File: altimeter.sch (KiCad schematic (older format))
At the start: 23 parts, among them J1 Conn_01x03_Male, J2 Conn_01x05_Male, J3 Conn_01x05_Male, J4 Conn_01x03_Male, Q1 Q_NMOS_DGS, U1 TLV760, U2 test, U3 accel, U4 RN4871, U5 EEPROM, U6 BMP280

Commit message: wip
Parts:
- removed C6: 1u, Capacitors_SMD:C_0805_HandSoldering, symbol CP
- removed J4: Conn_01x03_Male, Pin_Headers:Pin_Header_Straight_1x03_Pitch2.54mm, symbol Conn_01x03_Male
- removed Q1: Q_NMOS_DGS, TO_SOT_Packages_SMD:SOT-23, symbol Q_NMOS_DGS
- removed R4: 100k, Resistors_SMD:R_0805_HandSoldering, symbol R
- removed R5: 5, Resistors_SMD:R_0805_HandSoldering, symbol R
- removed U3: accel, SMD_Packages:SOIC-8-N, symbol accel
- removed U5: EEPROM, lib:SO8, symbol EEPROM
- C1, C2, C3, C4, C5, C7: footprint Capacitors_SMD:C_0805_HandSoldering -> Capacitors_SMD:C_0603
- J2, J3: footprint Pin_Headers:Pin_Header_Straight_1x05_Pitch2.54mm -> lib:pin5
- R1, R2, R3: footprint Resistors_SMD:R_0805_HandSoldering -> Resistors_SMD:R_0603
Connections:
- wire segments 119 -> 82

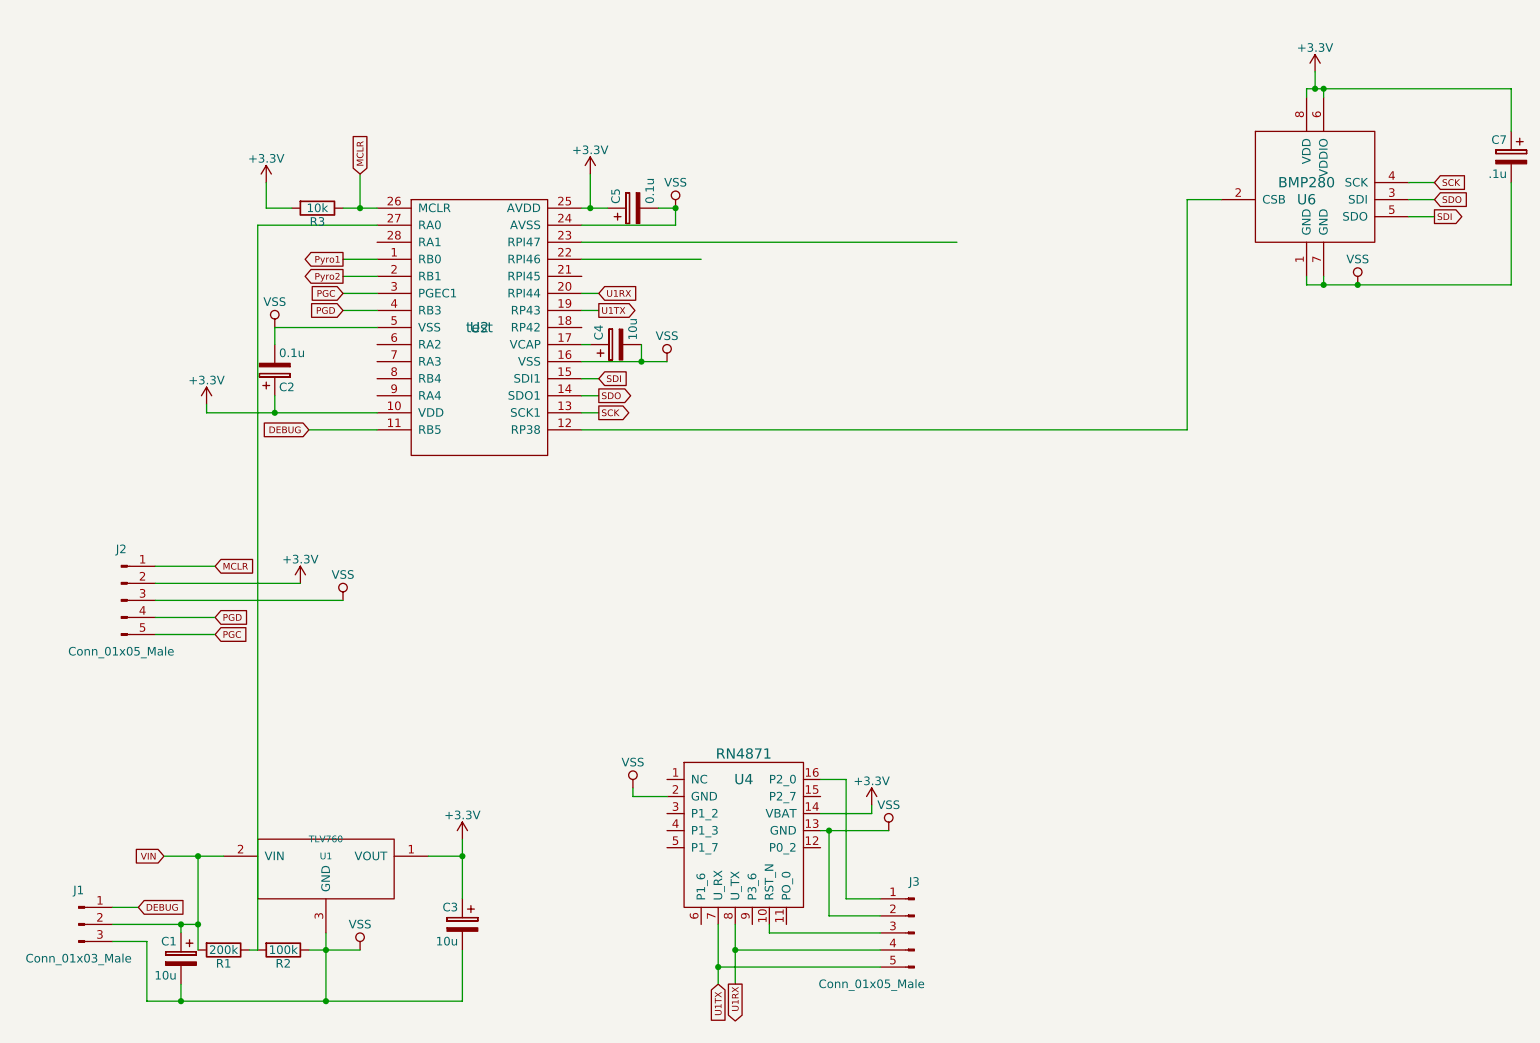
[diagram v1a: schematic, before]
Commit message: wip
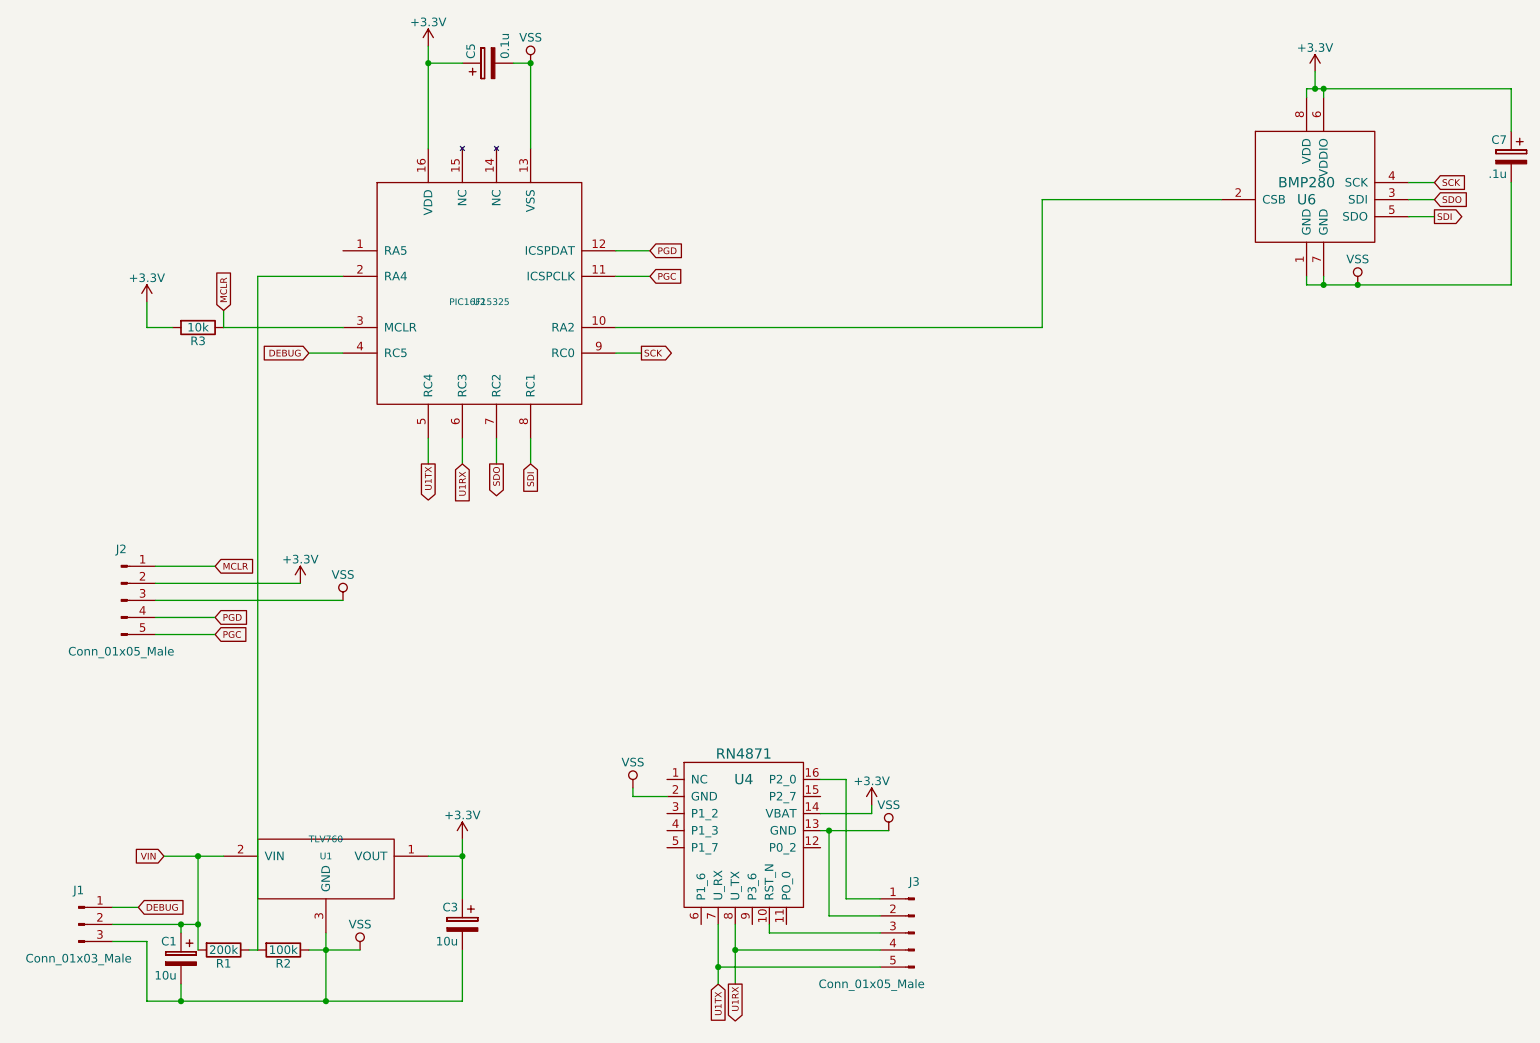
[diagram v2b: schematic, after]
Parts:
- removed C2: 0.1u, Capacitors_SMD:C_0603, symbol CP
- removed C4: 10u, Capacitors_SMD:C_0603, symbol CP
- removed U2: test, lib:QFN_28, symbol dsPIC33_qfn
- added U2: PIC16F15325, symbol PIC16F15325
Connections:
- net +3V3: now also U2.16 (VDD)
- net DEBUG: now also U2.4 (RC5)
- net MCLR: now also U2.3 (MCLR)
- net PGC: now also U2.11 (ICSPCLK)
- net PGD: now also U2.12 (ICSPDAT)
- net SCK: now also U2.9 (RC0)
- net SDI: now also U2.8 (RC1)
- net SDO: now also U2.7 (RC2)
- net U1RX: now also U2.6 (RC3)
- net U1TX: now also U2.5 (RC4)
- net VSS: now also U2.13 (VSS)
- net at U6.2 (CSB): now also U2.10 (RA2)
- net at R1.1, R2.2: now also U2.2 (RA4)
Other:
- moved on the sheet: C5, R3
